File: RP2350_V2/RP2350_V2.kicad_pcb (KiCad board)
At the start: 4 copper layers, 68.8 x 110.6 mm, 140 parts, among them IC1 DMP1045U-7, IC2 DMP1045U-7, IC3 DMP1045U-7, IC4 DMP1045U-7, J1 Conn_01x04_Pin, J3 USB_C_Receptacle_USB2.0_16P, J4 RF_CONNECTOR_5-1814832-2, J5 Conn_01x08_Socket, J6 Conn_01x02_Pin, J7 Conn_01x04_Pin, SW1 PTS 647 SN50 SMTR2 LFS, SW10 PTS 647 SN50 SMTR2 LFS, SW11 PTS 647 SN50 SMTR2 LFS, SW12 PTS 647 SN50 SMTR2 LFS, SW13 PTS 647 SN50 SMTR2 LFS, SW14 PTS 647 SN50 SMTR2 LFS, SW4 PTS 647 SN50 SMTR2 LFS, SW9 PTS 647 SN50 SMTR2 LFS, U1 RP2350_60QFN, U2 W25Q128JVS, U3 TPS62811QWRWYRQ1, U4 MCP73812T-420I-OT, U5 TLV3012AIDCKR, U6 74HC14, X1 ABM8-272-T3

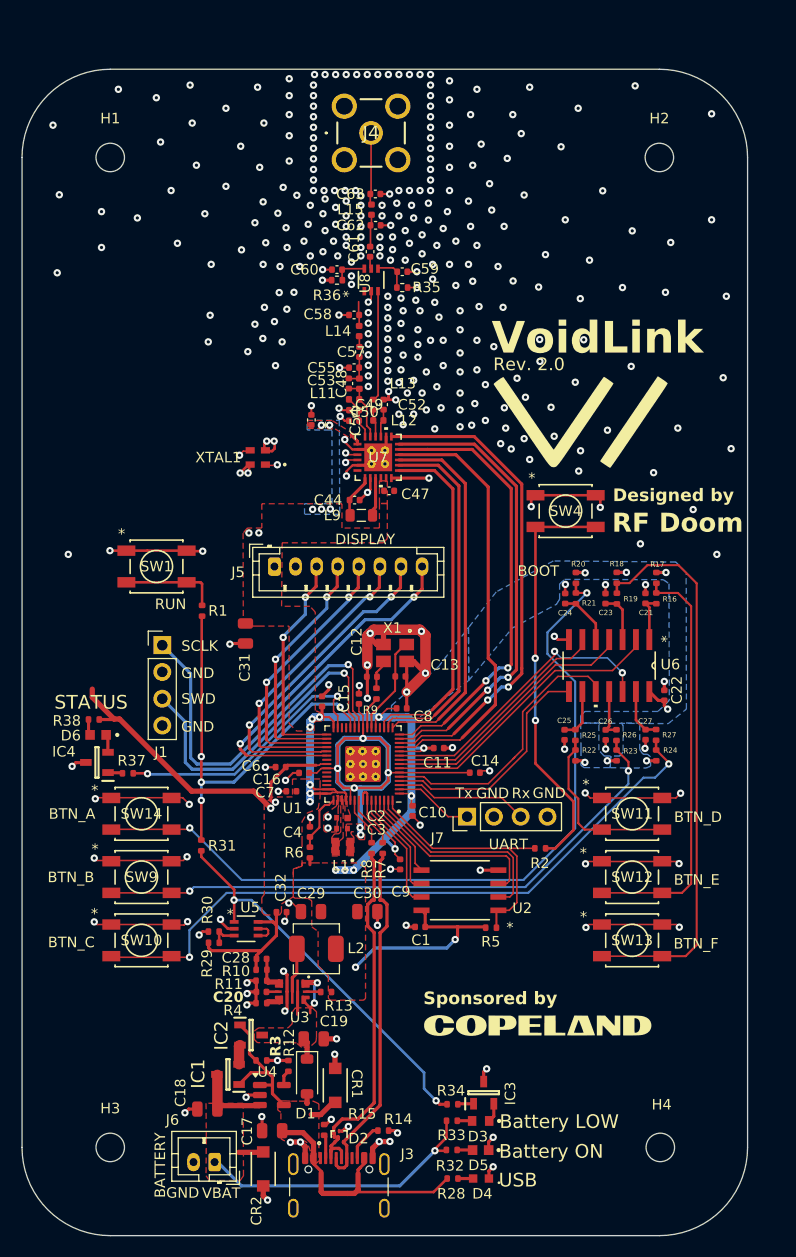
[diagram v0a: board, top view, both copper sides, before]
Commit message: Lots of Updatesgit add --allgit add --all
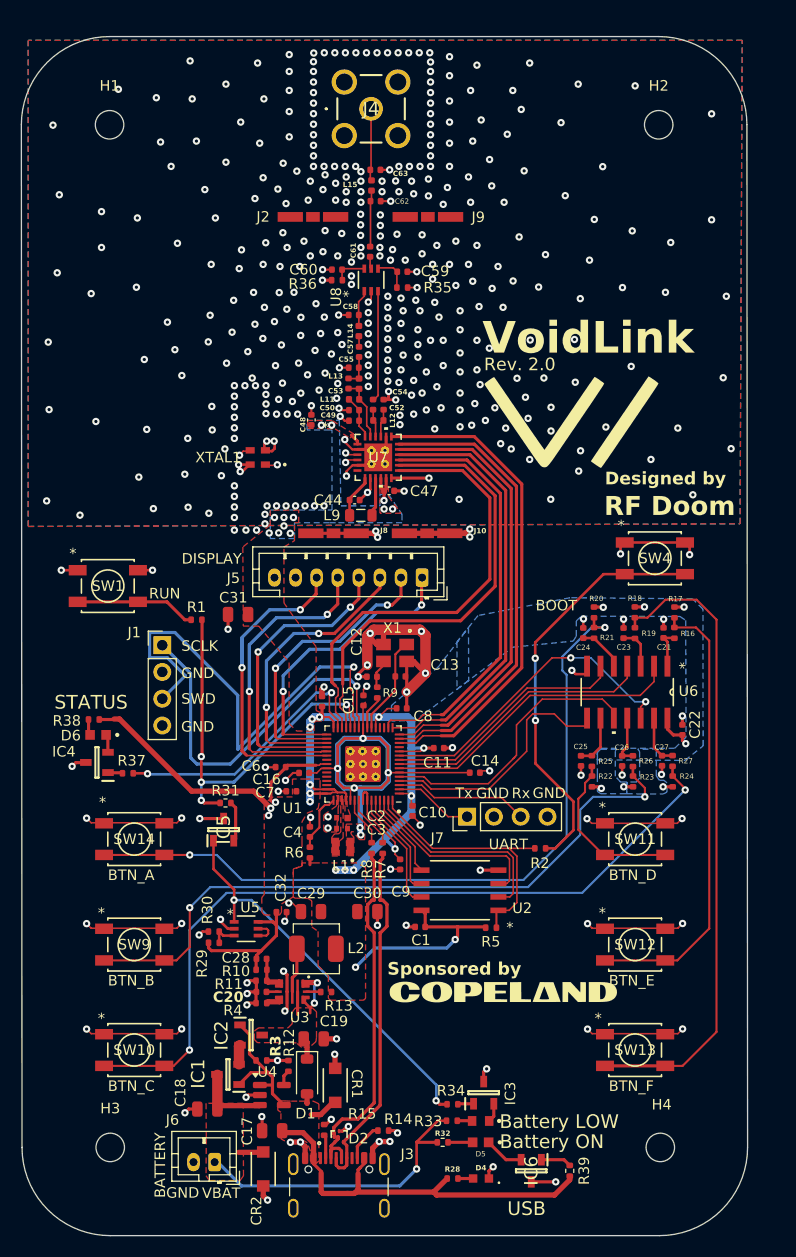
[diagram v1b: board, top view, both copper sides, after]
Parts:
- added IC5: DMP1045U-7, My_Footprints:SOT96P240X110-3N, F.Cu at (131.0, 110.6)
- added IC6: DMP1045U-7, My_Footprints:SOT96P240X110-3N, F.Cu at (160.2, 142.9)
- added J10: S0991-46R, My_Footprints:HARWIN_S0991-46R, F.Cu at (150.3, 82.5)
- added J2: S0991-46R, My_Footprints:HARWIN_S0991-46R, F.Cu at (139.4, 52.5)
- added J8: S0991-46R, My_Footprints:HARWIN_S0991-46R, F.Cu at (141.4, 82.5)
- added J9: S0991-46R, My_Footprints:HARWIN_S0991-46R, F.Cu at (150.3, 52.5)
- added R39: 100k, Resistor_SMD:R_0402_1005Metric, F.Cu at (163.8, 142.9)
- R28: value 86.6 -> 110
- R32: value 75 -> 91
- moved J5 14.0 mm to (149.8, 86.7), turned to 180 degrees
- moved SW10 10.4 mm to (122.5, 131.5)
- moved SW13 10.4 mm to (170.0, 131.5)
- moved SW4 9.58 mm to (171.9, 84.9)
- moved SW9 6.44 mm to (122.5, 121.5)
- moved SW12 6.41 mm to (170.0, 121.5)
- moved SW1 4.97 mm to (120.0, 87.5)
- moved R31 4.64 mm to (131.2, 108.1), turned to 0 degrees
- moved G*** 4.55 mm to (157.5, 126.0)
- moved C23 3.70 mm to (168.9, 92.0)
- moved C24 3.70 mm to (165.1, 92.0)
- moved R18 3.70 mm to (170.0, 90.0)
- moved C21 3.70 mm to (172.7, 91.9)
- moved R16 3.70 mm to (173.7, 91.9)
- moved R20 3.70 mm to (166.1, 90.0)
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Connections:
- D5 pad C: GND -> Net-(IC6-S)
- J5 pad 1: +3V3 -> /DISPLAY_BUSY
- J5 pad 2: GND -> /DISPLAY_RESET
- J5 pad 3: /DISPLAY_BUSY -> /DISPLAY_DC
- J5 pad 4: /DISPLAY_RESET -> /SPI1_CS
- J5 pad 5: /DISPLAY_DC -> /SPI1_CLK
- J5 pad 6: /SPI1_CS -> /SPI1_TX
- J5 pad 7: /SPI1_CLK -> GND
- J5 pad 8: /SPI1_TX -> +3V3
- R31 pad 1: /UVLO_RST -> /RUN
- R31 pad 2: /RUN -> Net-(IC5-S)
- U1 pad 12: SPIO_RX -> unconnected-(U1-GPIO8-Pad12)
- U1 pad 16: uC_RESET -> SPIO_RX
- U1 pad 17: uC_BUSY -> uC_RESET
- U1 pad 18: DIO1 -> unconnected-(U1-GPIO14-Pad18)
- U1 pad 27: unconnected-(U1-GPIO16-Pad27) -> uC_BUSY
- U1 pad 28: unconnected-(U1-GPIO17-Pad28) -> DIO1
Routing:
- net /SWD: track 31.7 -> 45.9 mm
- net VBUS: track 42.5 -> 56.4 mm
- net GND: track 195.4 -> 208.2 mm, vias 366 -> 442
- net Net-(R24-Pad2): track 64.8 -> 75.4 mm
- net DIO1: track 33.2 -> 43.5 mm
- net uC_BUSY: track 34.4 -> 43.7 mm
- net Net-(R18-Pad2): track 53.4 -> 61.3 mm
- net /DISPLAY_BUSY: track 21.0 -> 28.2 mm
- net Net-(R23-Pad2): track 58.0 -> 64.6 mm
- net uC_RESET: track 35.3 -> 40.2 mm
- net /DISPLAY_RESET: track 23.2 -> 27.9 mm
- net Net-(R20-Pad2): track 75.2 -> 70.9 mm
- net Net-(IC6-S): track 0.00 -> 3.86 mm
- net Net-(IC5-S): track 0.00 -> 3.84 mm
- net /BTN_MACRO_C: track 28.1 -> 31.4 mm
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- added copper zone on B.Cu, net GND
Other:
- board size 68.8 x 110.6 mm -> 68.9 x 113.7 mm

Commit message: optimizations, refinements
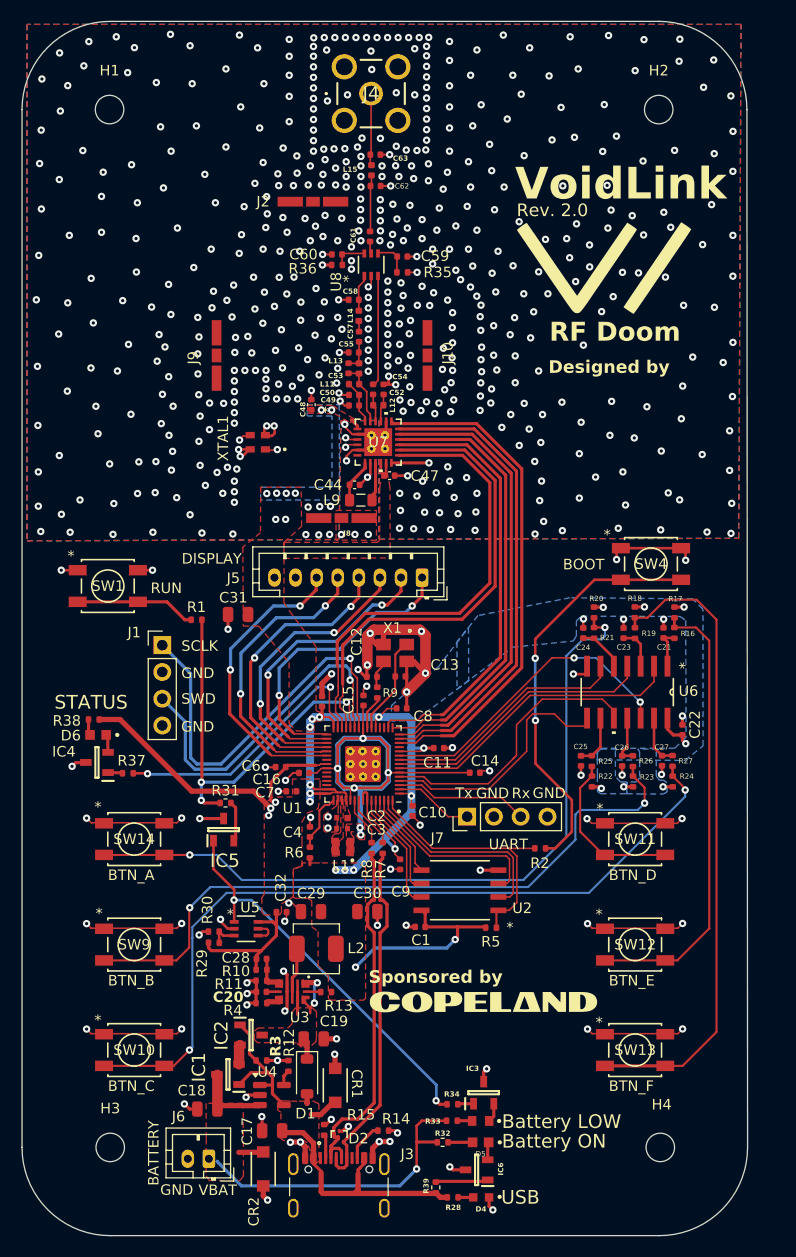
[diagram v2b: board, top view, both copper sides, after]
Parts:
- moved J9 24.0 mm to (130.3, 65.6), turned to 90 degrees
- moved J10 16.9 mm to (150.3, 65.6), turned to 90 degrees
- moved G*** 14.9 mm to (167.1, 57.4)
- moved R39 12.8 mm to (151.1, 144.5)
- moved IC6 5.18 mm to (155.0, 142.9), turned to 180 degrees
- moved G*** 2.10 mm to (155.6, 126.9)
- moved D4 1.79 mm to (155.4, 145.5)
- moved R28 1.79 mm to (152.7, 145.5)
- moved J8 1.63 mm to (142.2, 81.1)
- moved C47 1.44 mm to (146.7, 77.0)
- moved ? 1.44 mm to (146.3, 74.5)
- moved ? 1.44 mm to (145.0, 74.5)
- moved ? 1.44 mm to (145.0, 73.2)
- moved ? 1.44 mm to (146.3, 73.2)
- moved C48 1.44 mm to (139.3, 70.3)
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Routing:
- net VBUS: track 56.4 -> 42.3 mm
- net GND: track 208.2 -> 194.1 mm, vias 442 -> 618
- net /SWD: track 45.9 -> 32.7 mm
- net /SPI1_CLK: track 34.3 -> 28.6 mm
- net /SPI1_TX: track 32.1 -> 28.7 mm
- net /SWCLK: track 35.4 -> 38.2 mm
- net Net-(IC6-S): track 3.86 -> 1.79 mm
- net Net-(IC6-G): track 2.93 -> 5.00 mm
- net SPI0_TX: track 42.1 -> 43.7 mm
- net uC_BUSY: track 43.7 -> 45.3 mm
- net SPIO_RX: track 41.0 -> 42.6 mm
- net SPIO_CLK: track 43.8 -> 45.2 mm
- net uC_RESET: track 40.2 -> 41.6 mm
- net CS/NSS: track 46.2 -> 47.7 mm
- net /SX1262/DIO2: track 25.5 -> 26.8 mm
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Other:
- board size 68.9 x 113.7 mm -> 68.8 x 115.1 mm
